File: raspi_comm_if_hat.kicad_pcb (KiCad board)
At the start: 2 copper layers, 65 x 56 mm, 66 parts, among them J1 B04B-XA, J2 Conn_02x20_Odd_Even, J3 B04B-XA, J4 Conn_01x02, J5 Conn_01x04, J6 B04B-XA, Q1 Q_NMOS_GSD, Q2 Q_NMOS_GSD, Q3 Q_NMOS_GSD, Q4 Q_NMOS_GSD, Q5 Q_NMOS_GSD, SW2 SW_DIP_x02, U1 MCP25625-x-SS, U2 74AHC1G04, U3 74AHC1G04, U4 AP2171W, U5 AP2171W, U6 AP2331, U7 AP2331, U8 AP2171W, U9 AP2171W, Y1 16MHz

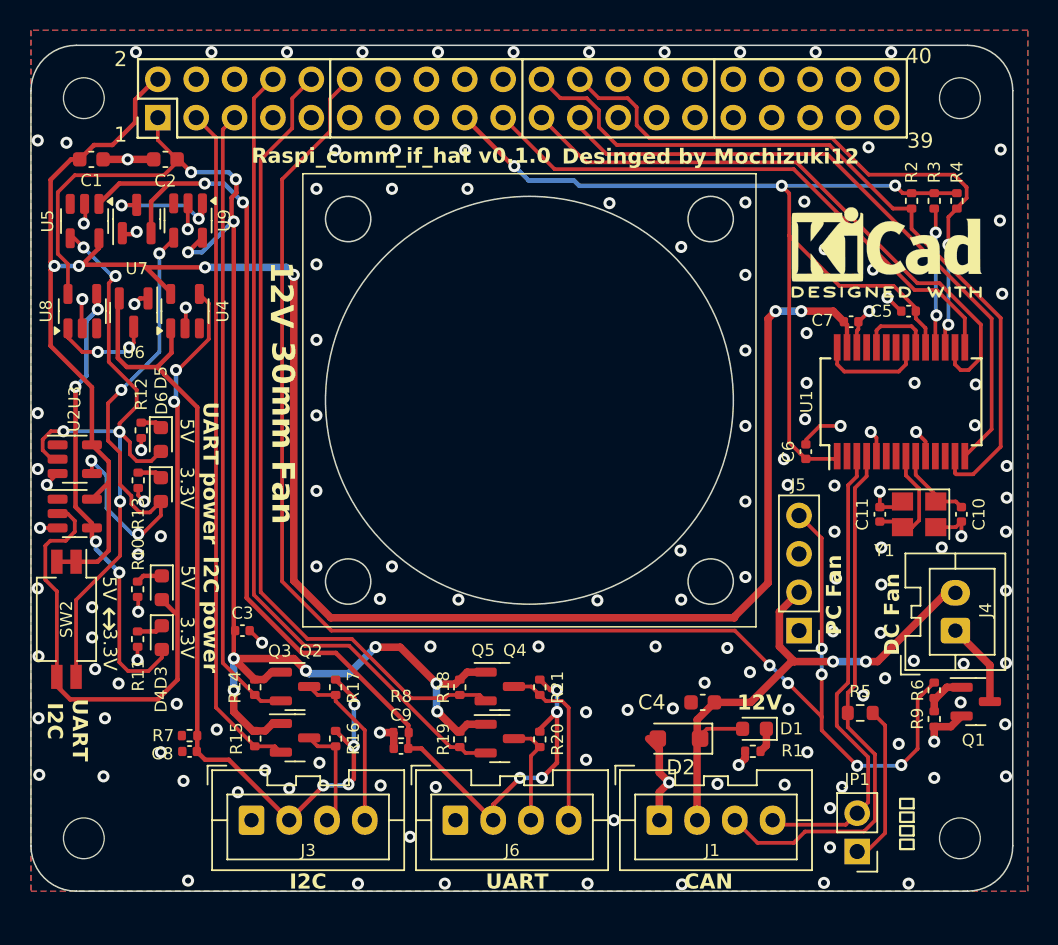
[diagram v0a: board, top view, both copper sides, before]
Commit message: v0.2.0 release
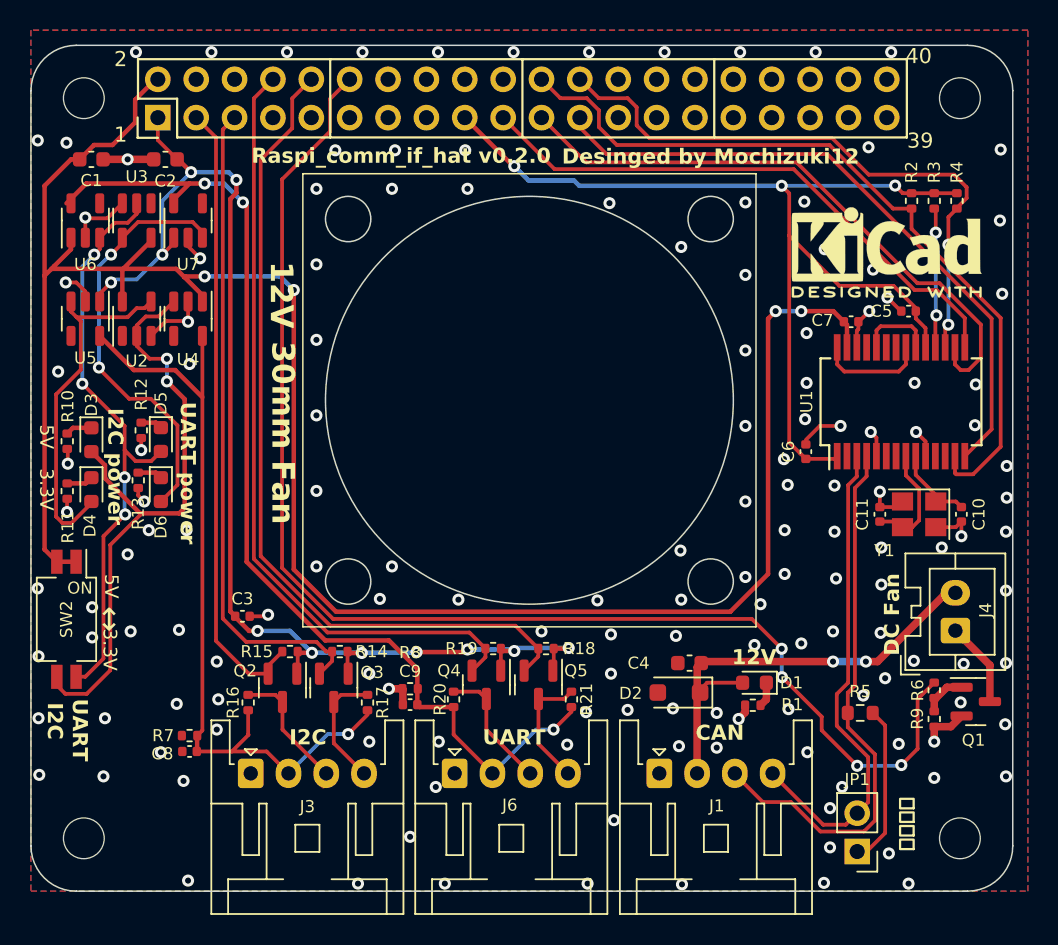
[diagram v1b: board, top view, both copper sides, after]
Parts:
- removed J5: Conn_01x04, Connector_PinHeader_2.54mm:PinHeader_1x04_P2.54mm_Vertical
- removed U8, U9: AP2171W, Package_TO_SOT_SMD:SOT-23-5
- J1, J3, J6: footprint Connector_JST:JST_XA_B04B-XASK-1_1x04_P2.50mm_Vertical -> Connector_JST:JST_XA_S04B-XASK-1_1x04_P2.50mm_Horizontal
- U4, U5: value AP2171W -> XC8110
- U6, U7: value AP2331 -> XC8110; footprint Package_TO_SOT_SMD:SOT-23 -> Package_TO_SOT_SMD:SOT-23-5
- moved U3 16.3 mm to (107.0, 65.6), turned to -90 degrees
- moved U2 13.5 mm to (107.0, 72.1), turned to 90 degrees
- moved D4 10.9 mm to (104.0, 83.4)
- moved D3 10.9 mm to (104.0, 80.1)
- moved R10 10.9 mm to (102.4, 80.2)
- moved R11 10.9 mm to (102.4, 83.5)
- moved U6 6.88 mm to (103.6, 65.6), turned to 90 degrees
- moved U5 6.46 mm to (103.6, 72.1)
- moved R19 6.41 mm to (130.6, 93.9), turned to 180 degrees
- moved R20 6.29 mm to (128.0, 97.3), turned to 90 degrees
- moved R16 6.26 mm to (114.4, 97.5), turned to 90 degrees
- moved R18 6.26 mm to (134.1, 93.9), turned to 180 degrees
- moved R15 6.22 mm to (117.2, 94.1), turned to 180 degrees
- moved R14 6.11 mm to (120.5, 94.1), turned to 180 degrees
- moved Q4 3.67 mm to (130.2, 96.3), turned to -90 degrees
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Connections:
- U4 pad 1: I2C_PWR -> +5V
- U4 pad 3: unconnected-(U4-~{FLG}-Pad3) -> Net-(D3-A)
- U4 pad 4: Net-(D3-A) -> unconnected-(U4-NC-Pad4)
- U4 pad 5: +5V -> I2C_PWR
- U5 pad 1: UART_PWR -> +3.3V
- U5 pad 3: unconnected-(U5-~{FLG}-Pad3) -> Net-(D4-A)
- U5 pad 4: Net-(D5-A) -> unconnected-(U5-NC-Pad4)
- U5 pad 5: +5V -> I2C_PWR
- U6 pad 1: GND -> +5V
- U6 pad 2: I2C_PWR -> GND
- U6 pad 3: Net-(U6-VI) -> Net-(D5-A)
- U7 pad 1: GND -> +3.3V
- U7 pad 2: UART_PWR -> GND
- U7 pad 3: Net-(U7-VI) -> Net-(D6-A)
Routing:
- net +3.3V: track 166.0 -> 152.5 mm, vias 13 -> 14
- net FAN_PWM: track 102.0 -> 88.6 mm, vias 6 -> 4
- net Net-(D3-A): track 51.5 -> 41.9 mm
- net UART_PWR: track 78.6 -> 70.3 mm, vias 6 -> 3
- net Net-(U7-VI): track 7.61 -> 0.00 mm, vias 2 -> 0
- net Net-(U6-VI): track 6.81 -> 0.00 mm, vias 2 -> 0
- net +12V: track 36.0 -> 29.5 mm
- net Net-(D4-A): track 30.2 -> 23.7 mm, vias 4 -> 0
- net I2C_PWR: track 58.6 -> 52.9 mm, vias 4 -> 1
- net Net-(D5-A): track 44.7 -> 39.2 mm, vias 5 -> 4
- net Net-(D6-A): track 32.7 -> 28.0 mm, vias 4 -> 2
- net GND: track 47.1 -> 42.9 mm, vias 150 -> 151
- net SDA: track 45.1 -> 41.4 mm
- net RX_conn: track 11.7 -> 8.11 mm
- net SDL_conn: track 11.1 -> 7.98 mm
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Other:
- board text added: "ON"
- board text added: "Raspi_comm_if_hat v0.2.0"
- board text removed: "PC Fan"
- board text removed: "Raspi_comm_if_hat v0.1.0"
